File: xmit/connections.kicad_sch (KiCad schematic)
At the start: 16 parts, among them J501 Conn_01x02, J502 Conn_01x02, J503 Conn_01x02, J504 Conn_01x02, J505 Conn_Coaxial, J506 Conn_01x02

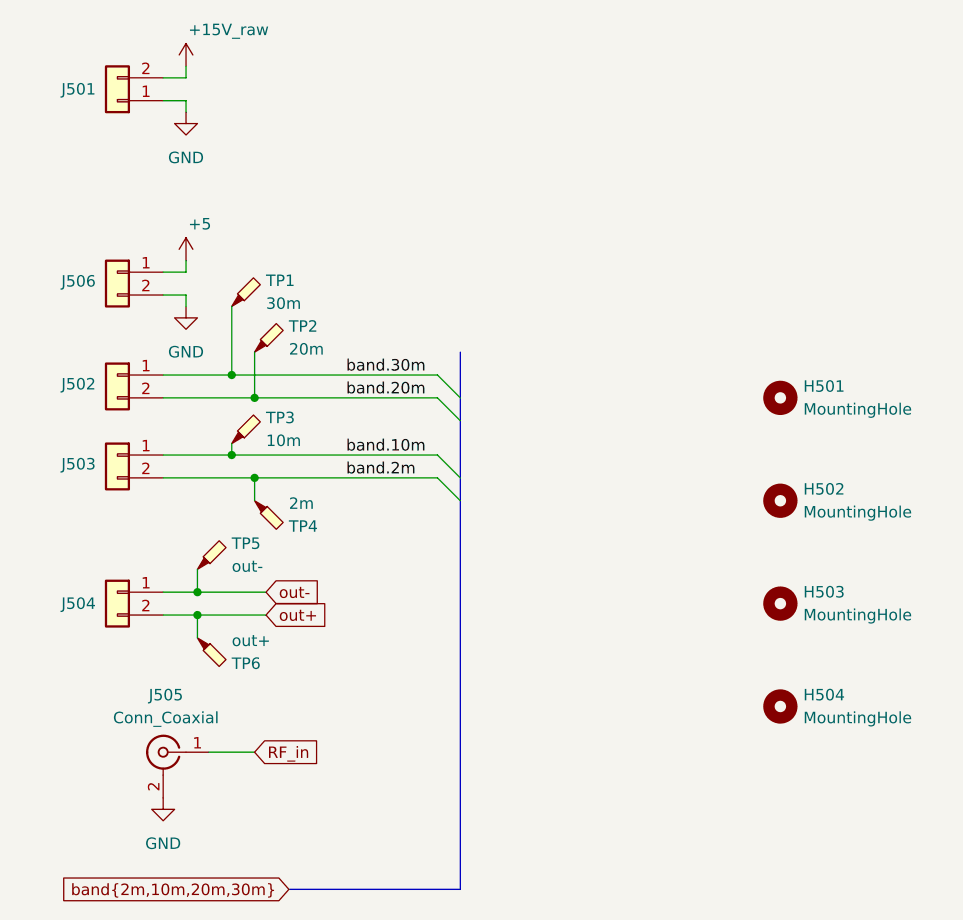
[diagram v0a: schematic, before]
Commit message: changes up to first spin
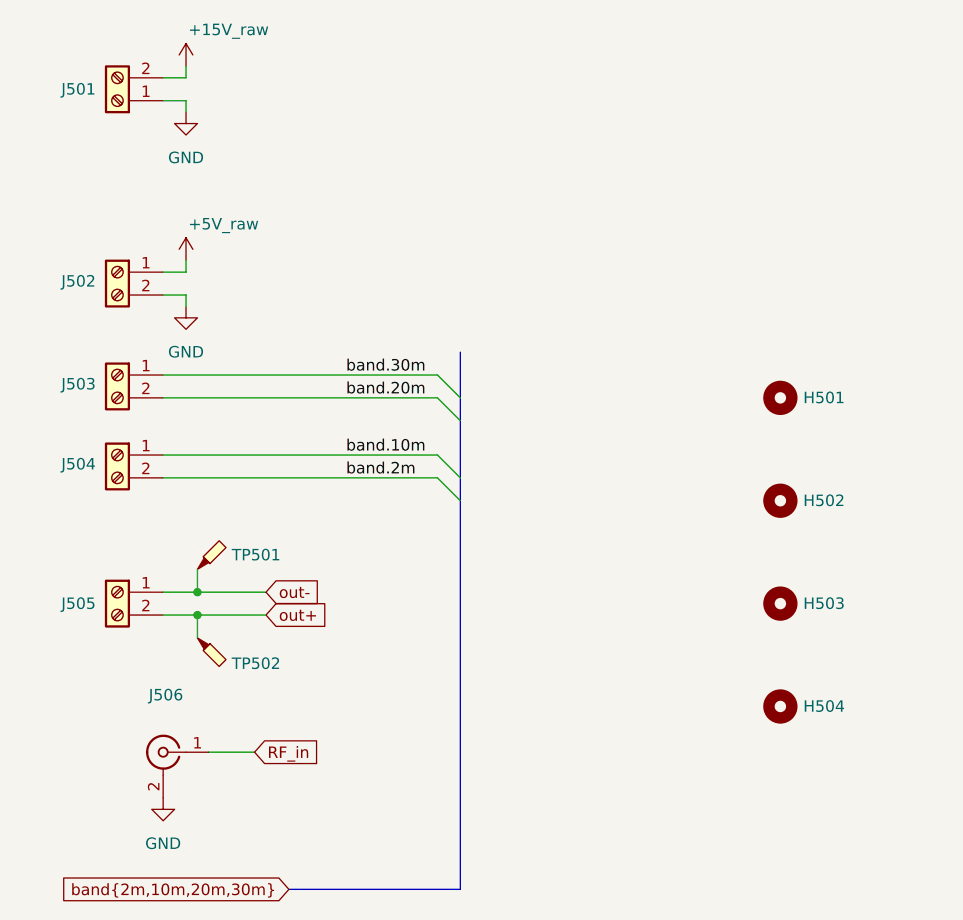
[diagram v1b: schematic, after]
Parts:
- removed TP1: 30m, TestPoint:TestPoint_Pad_1.0x1.0mm, symbol Connector:TestPoint_Probe
- removed TP2: 20m, TestPoint:TestPoint_Pad_1.0x1.0mm, symbol Connector:TestPoint_Probe
- removed TP3: 10m, TestPoint:TestPoint_Pad_1.0x1.0mm, symbol Connector:TestPoint_Probe
- removed TP4: 2m, TestPoint:TestPoint_Pad_1.0x1.0mm, symbol Connector:TestPoint_Probe
- H501, H502, H503, H504: value MountingHole -> (none); KiLib_Generator (none) -> mounting_hardware/mounting_hole
- J501: value Conn_01x02 -> (none); footprint Connector:terminal_block_02 -> TerminalBlock_TE-Connectivity:TerminalBlock_TE_282834-2_1x02_P2.54mm_Horizontal; symbol Connector_Generic:Conn_01x02 -> Connector:Screw_Terminal_01x02; KiLib_Generator (none) -> terminal_block/TE_Connectivity; now left out of the parts list
- J502: renamed from J506; value Conn_01x02 -> (none); footprint Connector:terminal_block_02 -> TerminalBlock_TE-Connectivity:TerminalBlock_TE_282834-2_1x02_P2.54mm_Horizontal; symbol Connector_Generic:Conn_01x02 -> Connector:Screw_Terminal_01x02; KiLib_Generator (none) -> terminal_block/TE_Connectivity; now left out of the parts list
- J503: renamed from J502; value Conn_01x02 -> (none); footprint Connector:terminal_block_02 -> TerminalBlock_TE-Connectivity:TerminalBlock_TE_282834-2_1x02_P2.54mm_Horizontal; symbol Connector_Generic:Conn_01x02 -> Connector:Screw_Terminal_01x02; KiLib_Generator (none) -> terminal_block/TE_Connectivity; now left out of the parts list
- J504: renamed from J503; value Conn_01x02 -> (none); footprint Connector:terminal_block_02 -> TerminalBlock_TE-Connectivity:TerminalBlock_TE_282834-2_1x02_P2.54mm_Horizontal; symbol Connector_Generic:Conn_01x02 -> Connector:Screw_Terminal_01x02; KiLib_Generator (none) -> terminal_block/TE_Connectivity; now left out of the parts list
- J505: renamed from J504; value Conn_01x02 -> (none); footprint Connector:terminal_block_02 -> TerminalBlock_TE-Connectivity:TerminalBlock_TE_282834-2_1x02_P2.54mm_Horizontal; symbol Connector_Generic:Conn_01x02 -> Connector:Screw_Terminal_01x02; KiLib_Generator (none) -> terminal_block/TE_Connectivity; now left out of the parts list
- J506: renamed from J505; value Conn_Coaxial -> (none); LCSC Part # (none) -> C49118400; now left out of the parts list
- TP501: renamed from TP5; value out- -> (none); LCSC Part # (none) -> C45367201; now left out of the parts list
- TP502: renamed from TP6; value out+ -> (none); LCSC Part # (none) -> C113518; now left out of the parts list
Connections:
- net +5 renamed +5V_raw
